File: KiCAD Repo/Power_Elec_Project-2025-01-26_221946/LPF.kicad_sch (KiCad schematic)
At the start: 2 parts, among them U1 LM358

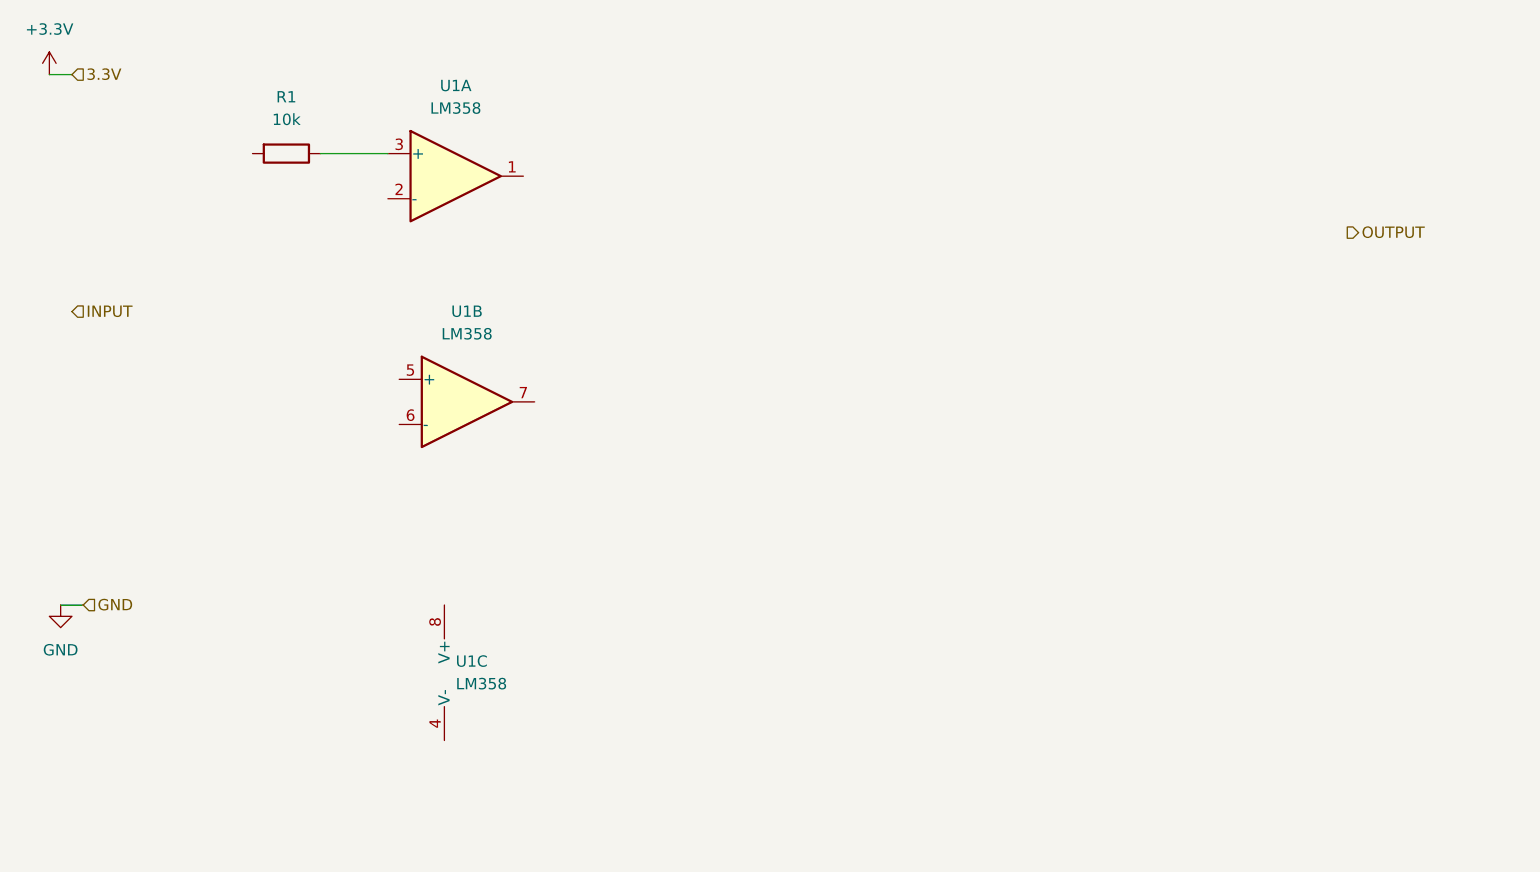
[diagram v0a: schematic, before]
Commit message: LPF design
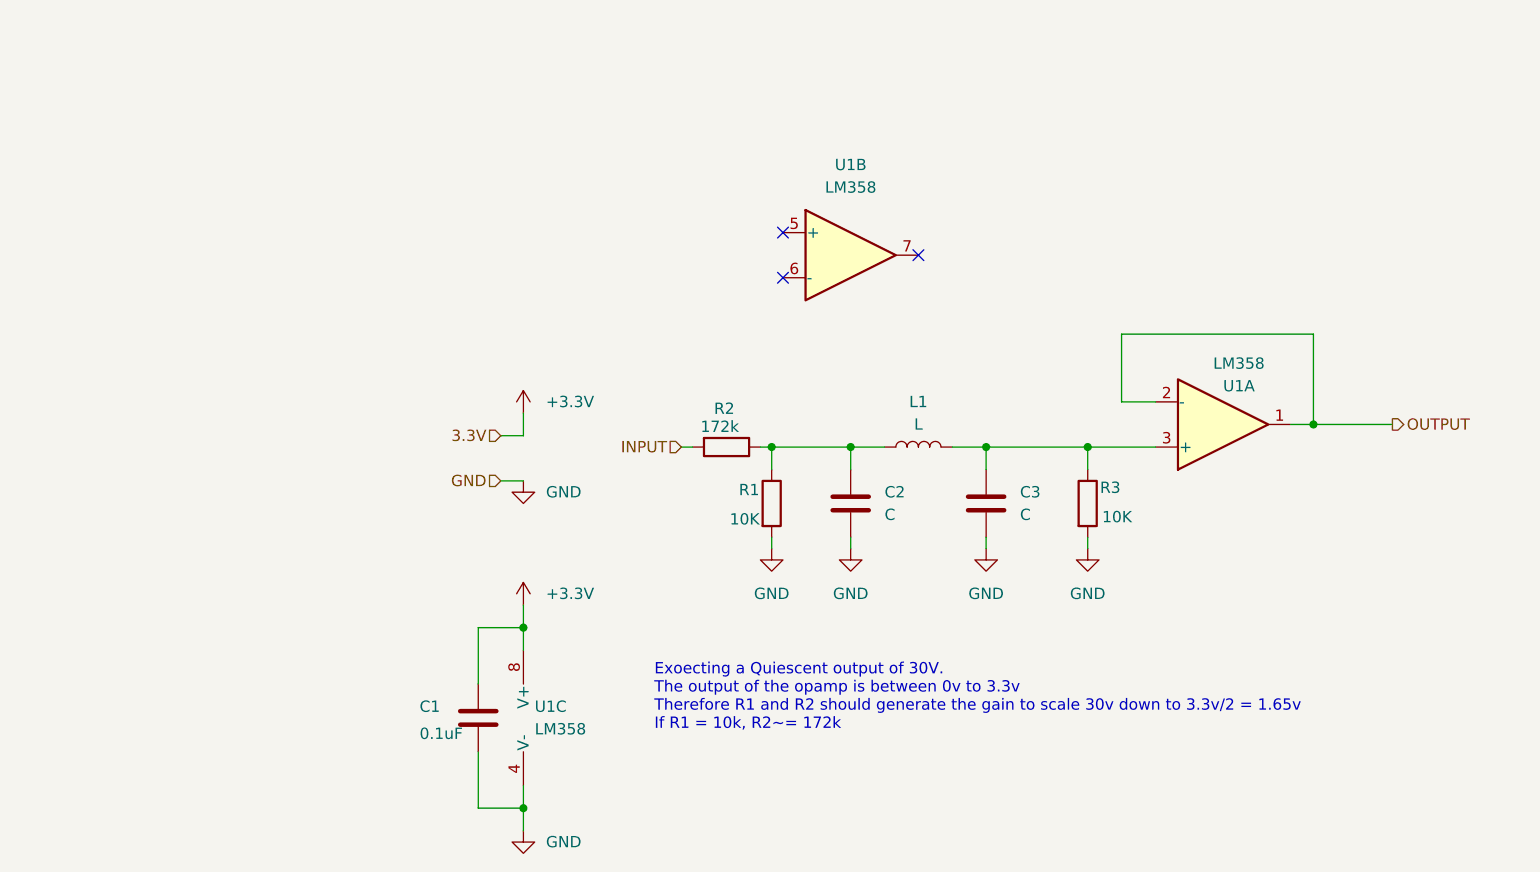
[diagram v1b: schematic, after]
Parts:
- added C1: 0.1uF, symbol Device:C
- added C2, C3: C, symbol Device:C
- added L1: L, symbol Device:L
- added R2: 172k, Resistor_SMD:R_0603_1608Metric, symbol Device:R
- added R3: 10K, Resistor_SMD:R_0805_2012Metric, symbol Device:R
- R1: value 10k -> 10K
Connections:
- net +3.3V: now also U1.8 (V+), C1.1
- net GND: now also R1.2, U1.4 (V-), C1.2, C2.2, C3.2, R3.2
- net INPUT: now also R2.2
- net OUTPUT: now also U1.1, U1.2 (-)
- net at U1.3 (+): now also C3.1, L1.2, R3.1; no longer R1.1
- new net: C2.1, L1.1, R1.1, R2.1
- no-connect marks 0 -> 3
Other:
- note added: "Exoecting a Quiescent output of 30V. The output of the opamp is between 0v to 3.3v Therefore R1 and R2 should generate the gain to scale 30v down to 3.3v/2 = 1.65v If R1 = 10k, R2~= 172k"
- moved on the sheet: R1, U1A, U1B, U1C
